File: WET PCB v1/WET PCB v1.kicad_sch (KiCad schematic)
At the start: 25 parts, among them J1 XT60, J2 XT60 or Terminal, J3 Conn_01x02_Pin, Q101 Q_NMOS_Depletion_GDS, Q102 Q_NMOS_Depletion_GDS, Q201 Q_NMOS_Depletion_GDS, Q202 Q_NMOS_Depletion_GDS, Q203 Q_NMOS_Depletion_GDS, Q204 Q_NMOS_Depletion_GDS, U3 Opamp_Dual

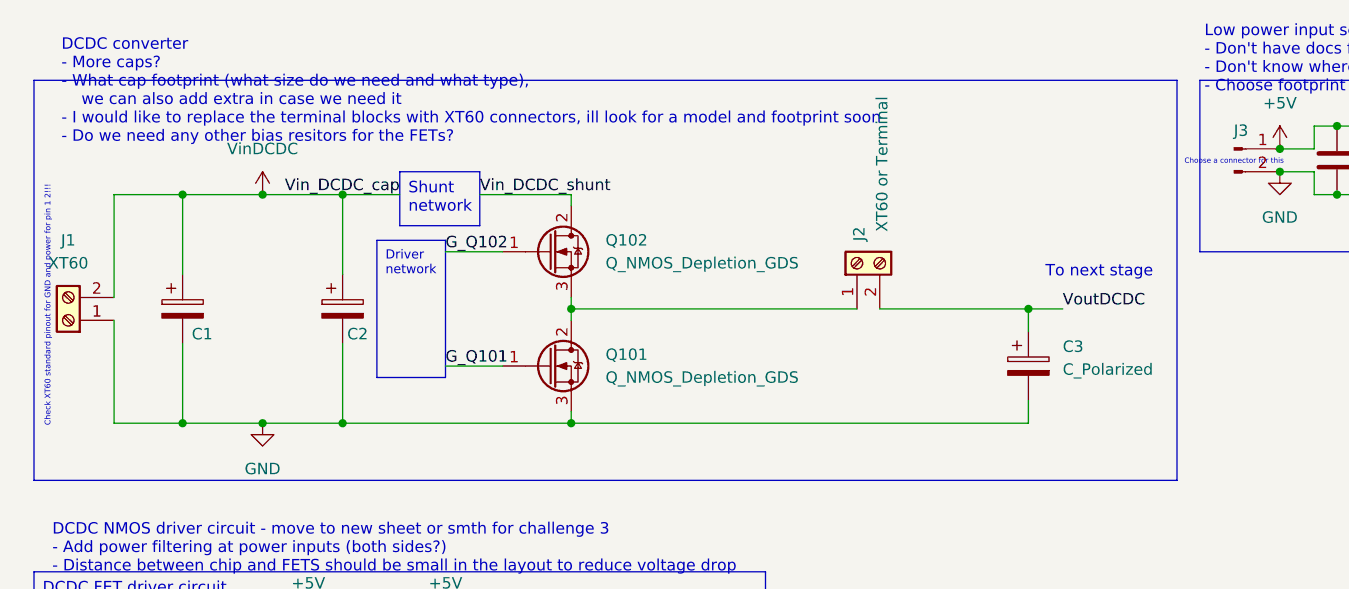
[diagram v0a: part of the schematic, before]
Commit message: Jake update friday
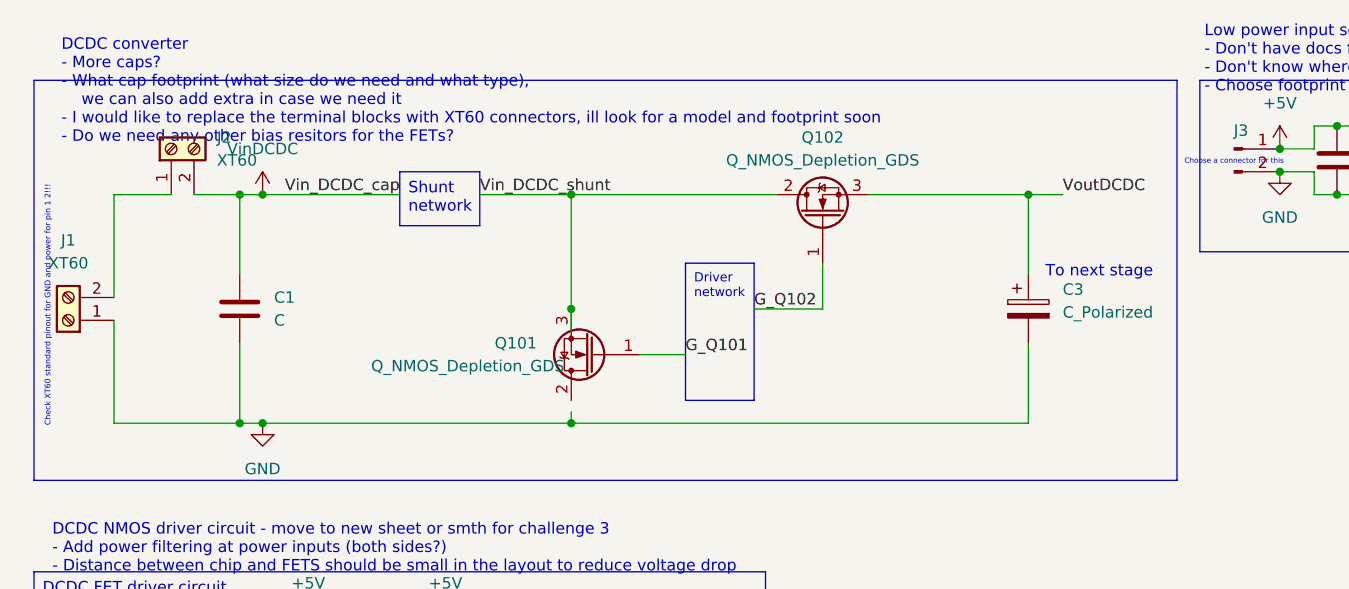
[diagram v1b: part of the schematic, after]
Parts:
- removed C1, C2: C_Polarized, symbol Device:C_Polarized
- added C1: C, symbol Device:C
- J2: value XT60 or Terminal -> XT60
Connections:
- net GND: now also C1.2; no longer Q101.3 (S)
- net VinDCDC: now also J2.2 (Pin_2), C1.1; no longer J1.2 (Pin_2)
- net Vin_DCDC_shunt: now also Q101.3 (S)
- net VoutDCDC: now also Q102.3 (S); no longer J2.2 (Pin_2)
- new net: J1.2 (Pin_2), J2.1 (Pin_1)
- now unconnected: Q101.2 (D)
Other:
- moved on the sheet: C3, Q101, Q102
